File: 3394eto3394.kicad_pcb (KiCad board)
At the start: 2 copper layers, 21.5 x 31.2 mm, 11 parts, among them J1 Conn_01x20_Male, J2 Conn_01x02_Male, J3 Conn_01x02_Male, J4 Conn_01x02_Male, U1 AS3394E

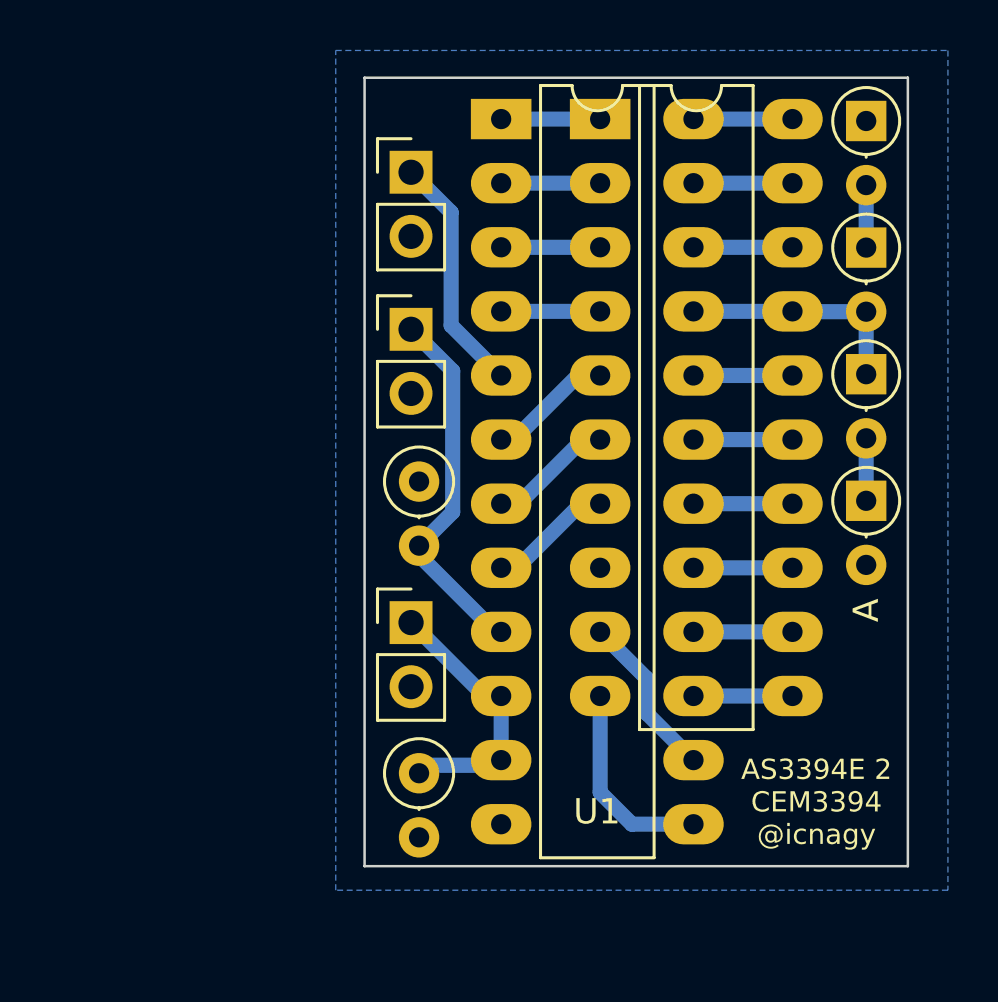
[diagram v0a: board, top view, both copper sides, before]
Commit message: Version 2
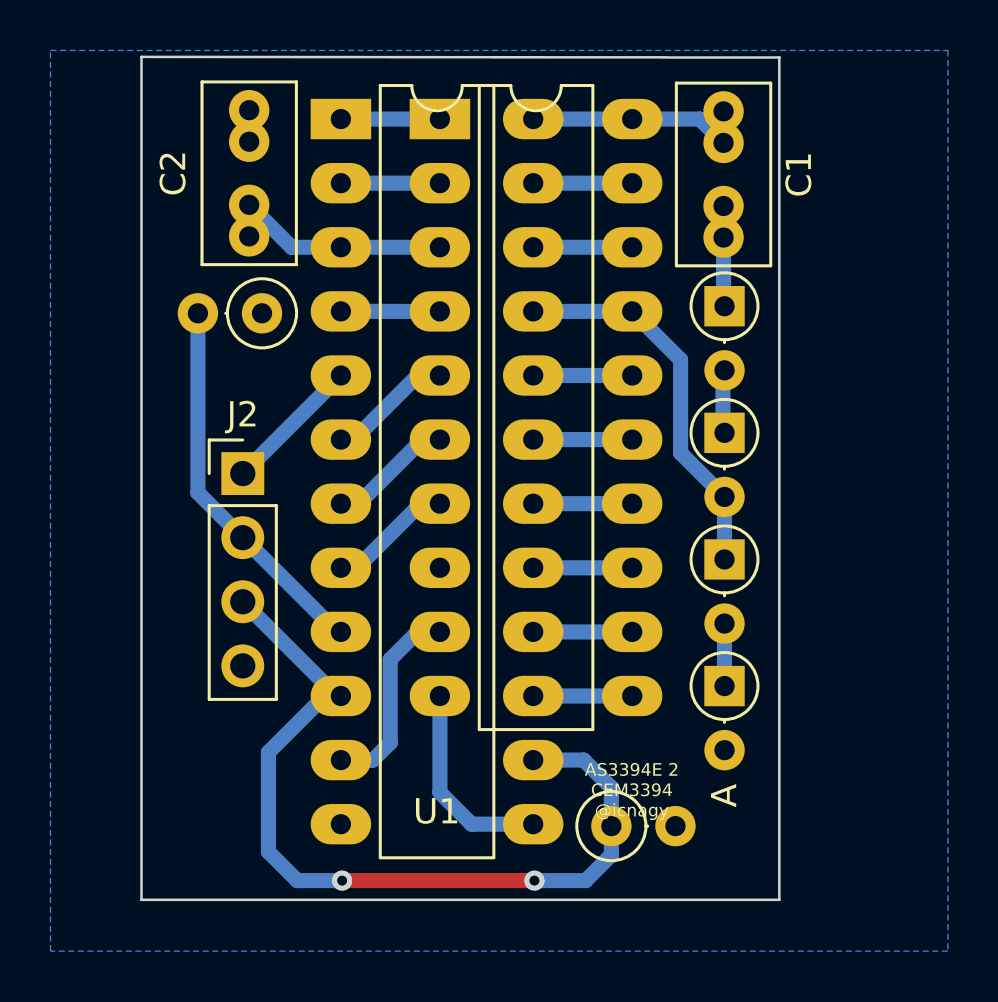
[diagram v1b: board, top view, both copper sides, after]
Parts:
- removed J3, J4: Conn_01x02_Male, Connector_PinHeader_2.54mm:PinHeader_1x02_P2.54mm_Vertical
- added C1: 100n, Capacitor_THT:C_Rect_L7.0mm_W3.5mm_P2.50mm_P5.00mm, F.Cu at (57.1, 29.5)
- added C2: 100n, Capacitor_THT:C_Rect_L7.0mm_W3.5mm_P2.50mm_P5.00mm, F.Cu at (38.4, 34.4)
- J2: value Conn_01x02_Male -> Conn_01x04_Male; footprint Connector_PinHeader_2.54mm:PinHeader_1x02_P2.54mm_Vertical -> Connector_PinHeader_2.54mm:PinHeader_1x04_P2.54mm_Vertical
- R3: value 1k -> 500R
- moved J2 13.7 mm to (38.1, 43.8)
- moved D1 9.24 mm to (57.2, 42.2)
- moved D2 9.24 mm to (57.2, 37.2)
- moved D3 9.24 mm to (57.2, 47.2)
- moved D4 9.24 mm to (57.2, 52.2)
- moved R1 9.12 mm to (38.9, 37.5), turned to 180 degrees
- moved R3 7.90 mm to (52.7, 57.8), turned to 0 degrees
- moved J1 6.35 mm to (45.9, 29.8)
- moved U1 6.35 mm to (42.0, 29.8)
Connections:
- J1 pad 9: /EXT_IN -> /NOISE_IN
- J2 pad 2: GND -> /SAW_OUT
- U1 pad 11: /EXT_IN1 -> /NOISE_IN
- U1 pad 14: /EXT_IN -> /EXT_IN1
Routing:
- net /EXT_IN1: track 10.8 -> 33.9 mm, vias 0 -> 2
- net /NOISE_IN: track 0.00 -> 7.96 mm
- net /EXT_IN: track 6.61 -> 0.00 mm
- net /Cs: track 9.33 -> 15.3 mm
- net -VSW: track 3.92 -> 9.50 mm
- net +VSW: track 3.92 -> 9.18 mm
- net /SUB_OUT: track 9.53 -> 5.50 mm
- net GND: track 0.00 -> 2.74 mm
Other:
- board size 21.5 x 31.2 mm -> 25.3 x 33.4 mm
